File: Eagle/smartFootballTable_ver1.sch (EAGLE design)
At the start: 22 parts, among them IC1 LM2940CT, K1 ARK500/2

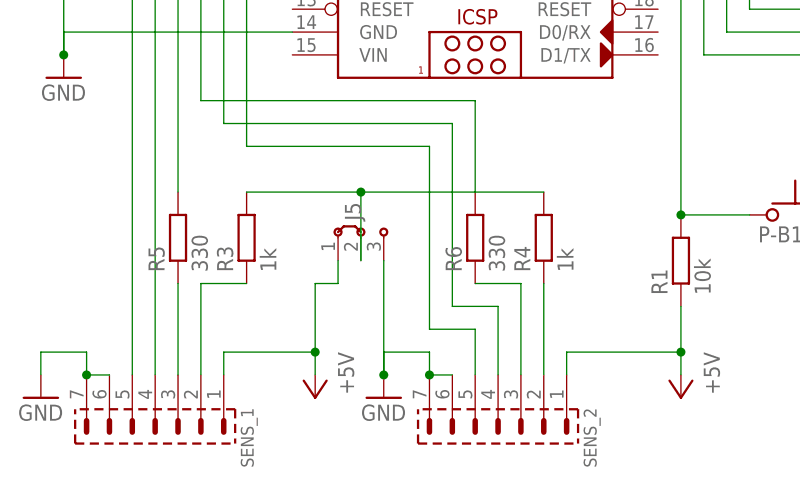
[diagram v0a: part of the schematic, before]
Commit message: Updated board with latest changes after soldering
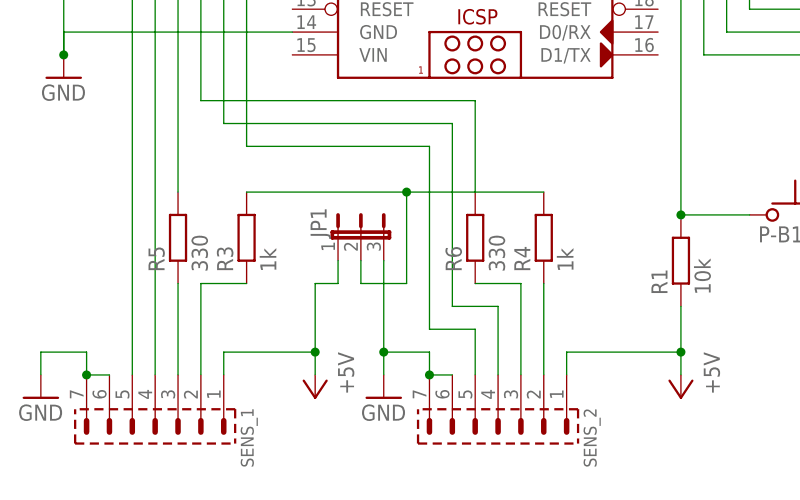
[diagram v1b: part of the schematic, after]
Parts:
- removed J5: (no value), jumper:J2X2MM
- added JP1: (no value), jumper:JP2W
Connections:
- net +5V: now also JP1.1; no longer J5.1
- net GND: now also JP1.3; no longer J5.3
- net N$31: now also JP1.2; no longer J5.2
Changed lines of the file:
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@@
 </part>
 <part name="ARDUINO_NANO1" library="ArduinoNanoV30" deviceset="ARDUINO_NANO" device=""/>
-<part name="J5" library="jumper" deviceset="J2" device="X2MM"/>
 <part name="DIS_1" library="#PaJa_konektory" deviceset="PSH02-07" device="W"/>
 <part name="DIS_2" library="#PaJa_konektory" deviceset="PSH02-07" device="W"/>
@@
 <part name="TEST" library="#PaJa_prepinace" deviceset="P-B1720" device=""/>
 <part name="J1" library="con-jack" deviceset="JACK-PLUG" device="1"/>
+<part name="JP1" library="jumper" deviceset="JP2W" device=""/>
 </parts>
 <sheets>
@@
 </instance>
 <instance part="ARDUINO_NANO1" gate="G$1" x="-7.62" y="53.34" rot="R180"/>
-<instance part="J5" gate="G$1" x="-20.32" y="10.16" rot="R90"/>
 <instance part="DIS_1" gate="KON" x="55.88" y="71.12" rot="R270"/>
 <instance part="DIS_2" gate="KON" x="55.88" y="35.56" rot="R270"/>
@@
 <instance part="TEST" gate="TLAC" x="27.94" y="12.7"/>
 <instance part="J1" gate="G$1" x="-45.72" y="111.76"/>
+<instance part="JP1" gate="1" x="-20.32" y="10.16"/>
 </instances>
 <busses>
@@
 <wire x1="-12.7" y1="-2.54" x2="-12.7" y2="-5.08" width="0.1524" layer="91"/>
 <wire x1="-12.7" y1="-5.08" x2="-10.16" y2="-5.08" width="0.1524" layer="91"/>
-<pinref part="J5" gate="G$1" pin="3"/>
-<wire x1="-17.78" y1="7.62" x2="-17.78" y2="-5.08" width="0.1524" layer="91"/>
-<junction x="-17.78" y="-5.08"/>
 <pinref part="SENS_2" gate="KON" pin="6"/>
 <pinref part="SENS_2" gate="KON" pin="7"/>
 <junction x="-12.7" y="-5.08"/>
+<pinref part="JP1" gate="1" pin="3"/>
+<wire x1="-17.78" y1="7.62" x2="-17.78" y2="-2.54" width="0.1524" layer="91"/>
+<junction x="-17.78" y="-2.54"/>
 </segment>
 </net>
@@
 <wire x1="-25.4" y1="-2.54" x2="-25.4" y2="5.08" width="0.1524" layer="91"/>
 <wire x1="-25.4" y1="5.08" x2="-22.86" y2="5.08" width="0.1524" layer="91"/>
-<pinref part="J5" gate="G$1" pin="1"/>
-<wire x1="-22.86" y1="5.08" x2="-22.86" y2="7.62" width="0.1524" layer="91"/>
 <wire x1="-35.56" y1="-5.08" x2="-35.56" y2="-2.54" width="0.1524" layer="91"/>
 <wire x1="-35.56" y1="-2.54" x2="-25.4" y2="-2.54" width="0.1524" layer="91"/>
 <junction x="-25.4" y="-2.54"/>
 <pinref part="SENS_1" gate="KON" pin="1"/>
+<pinref part="JP1" gate="1" pin="1"/>
+<wire x1="-22.86" y1="5.08" x2="-22.86" y2="7.62" width="0.1524" layer="91"/>
 </segment>
 </net>
@@
 <pinref part="R3" gate="G$1" pin="2"/>
 <pinref part="R4" gate="G$1" pin="2"/>
-<wire x1="-33.02" y1="15.24" x2="-20.32" y2="15.24" width="0.1524" layer="91"/>
-<pinref part="J5" gate="G$1" pin="2"/>
-<wire x1="-20.32" y1="15.24" x2="0" y2="15.24" width="0.1524" layer="91"/>
-<wire x1="-20.32" y1="7.62" x2="-20.32" y2="15.24" width="0.1524" layer="91"/>
-<junction x="-20.32" y="15.24"/>
-</segment>
-</net>
+<wire x1="-33.02" y1="15.24" x2="-15.24" y2="15.24" width="0.1524" layer="91"/>
+<pinref part="JP1" gate="1" pin="2"/>
+<wire x1="-15.24" y1="15.24" x2="0" y2="15.24" width="0.1524" layer="91"/>
+<wire x1="-20.32" y1="7.62" x2="-20.32" y2="5.08" width="0.1524" layer="91"/>
+<wire x1="-20.32" y1="5.08" x2="-15.24" y2="5.08" width="0.1524" layer="91"/>
+<wire x1="-15.24" y1="5.08" x2="-15.24" y2="15.24" width="0.1524" layer="91"/>
+<junction x="-15.24" y="15.24"/>
+</segment>
+</net>
